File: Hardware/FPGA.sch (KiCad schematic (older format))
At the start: 4 parts

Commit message: Getting down structure, some components created.
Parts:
- removed U? (x4): ICE40UP5K-SG48ITR, Package_DFN_QFN:QFN-48-1EP_7x7mm_P0.5mm_EP5.6x5.6mm, symbol FPGA_Lattice:ICE40UP5K-SG48ITR
- added U501: ICE40UP5K-SG48, tomu-fpga:QFN-48-1EP_7x7mm_P0.5mm_EP5.6x5.6mm, symbol pkl_lattice:ICE40UP5K-SG48
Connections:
- net labels added: LED_B, LED_G, LED_R
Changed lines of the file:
@@
 $EndDescr
 $Comp
-L FPGA_Lattice:ICE40UP5K-SG48ITR U?
-U 1 1 6121B3F0
-P 4200 2800
-F 0 "U?" H 4530 2853 50  0000 L CNN
-F 1 "ICE40UP5K-SG48ITR" H 4530 2762 50  0000 L CNN
-F 2 "Package_DFN_QFN:QFN-48-1EP_7x7mm_P0.5mm_EP5.6x5.6mm" H 4200 1450 50  0001 C CNN
-F 3 "http://www.latticesemi.com/Products/FPGAandCPLD/iCE40Ultra" H 3800 3800 50  0001 C CNN
-	1    4200 2800
+L pkl_lattice:ICE40UP5K-SG48 U501
+U 1 1 61224EB1
+P 6450 3150
+F 0 "U501" H 6450 5315 50  0000 C CNN
+F 1 "ICE40UP5K-SG48" H 6450 5224 50  0000 C CNN
+F 2 "tomu-fpga:QFN-48-1EP_7x7mm_P0.5mm_EP5.6x5.6mm" H 8750 3350 50  0001 C CNN
+F 3 "" H 8750 3350 50  0001 C CNN
+	1    6450 3150
 	1    0    0    -1
 $EndComp
-$Comp
-L FPGA_Lattice:ICE40UP5K-SG48ITR U?
-U 2 1 6121C11C
-P 6200 2850
-F 0 "U?" H 6200 1775 50  0000 C CNN
-F 1 "ICE40UP5K-SG48ITR" H 6200 1684 50  0000 C CNN
-F 2 "Package_DFN_QFN:QFN-48-1EP_7x7mm_P0.5mm_EP5.6x5.6mm" H 6200 1500 50  0001 C CNN
-F 3 "http://www.latticesemi.com/Products/FPGAandCPLD/iCE40Ultra" H 5800 3850 50  0001 C CNN
-	2    6200 2850
-	1    0    0    -1
-$EndComp
-$Comp
-L FPGA_Lattice:ICE40UP5K-SG48ITR U?
-U 3 1 6121CDD3
-P 7600 4600
-F 0 "U?" H 7930 4703 50  0000 L CNN
-F 1 "ICE40UP5K-SG48ITR" H 7930 4612 50  0000 L CNN
-F 2 "Package_DFN_QFN:QFN-48-1EP_7x7mm_P0.5mm_EP5.6x5.6mm" H 7600 3250 50  0001 C CNN
-F 3 "http://www.latticesemi.com/Products/FPGAandCPLD/iCE40Ultra" H 7200 5600 50  0001 C CNN
-	3    7600 4600
-	1    0    0    -1
-$EndComp
-$Comp
-L FPGA_Lattice:ICE40UP5K-SG48ITR U?
-U 4 1 6121D881
-P 5450 5350
-F 0 "U?" H 5680 5396 50  0000 L CNN
-F 1 "ICE40UP5K-SG48ITR" H 5680 5305 50  0000 L CNN
-F 2 "Package_DFN_QFN:QFN-48-1EP_7x7mm_P0.5mm_EP5.6x5.6mm" H 5450 4000 50  0001 C CNN
-F 3 "http://www.latticesemi.com/Products/FPGAandCPLD/iCE40Ultra" H 5050 6350 50  0001 C CNN
-	4    5450 5350
-	1    0    0    -1
-$EndComp
+Text HLabel 7450 3050 2    50   Output ~ 0
+LED_B
+Text HLabel 7450 2850 2    50   Output ~ 0
+LED_G
+Text HLabel 7450 2950 2    50   Output ~ 0
+LED_R
 $EndSCHEMATC

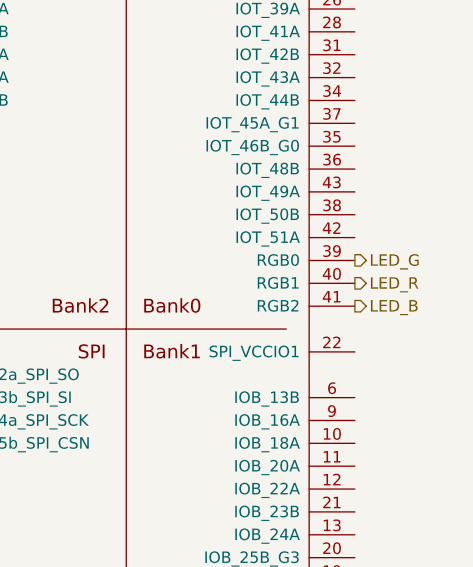
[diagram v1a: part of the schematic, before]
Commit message: Checking in some libraries.
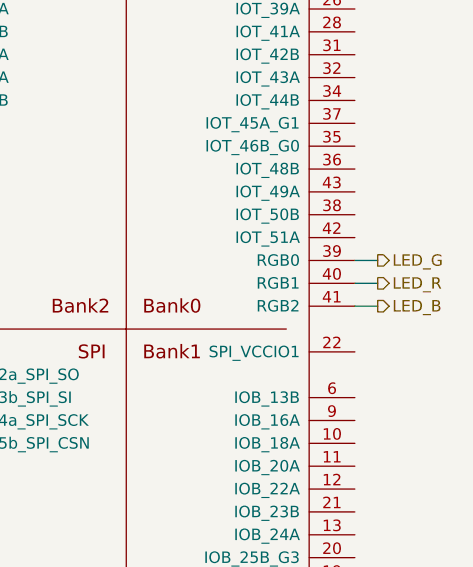
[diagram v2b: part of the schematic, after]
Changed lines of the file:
@@
 	1    0    0    -1
 $EndComp
-Text HLabel 7450 3050 2    50   Output ~ 0
+Text HLabel 7550 3050 2    50   Output ~ 0
 LED_B
-Text HLabel 7450 2850 2    50   Output ~ 0
+Text HLabel 7550 2850 2    50   Output ~ 0
 LED_G
-Text HLabel 7450 2950 2    50   Output ~ 0
+Text HLabel 7550 2950 2    50   Output ~ 0
 LED_R
+Wire Wire Line
+	7450 2850 7550 2850
+Wire Wire Line
+	7450 2950 7550 2950
+Wire Wire Line
+	7450 3050 7550 3050
 $EndSCHEMATC
